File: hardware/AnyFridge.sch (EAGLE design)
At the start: 12 parts

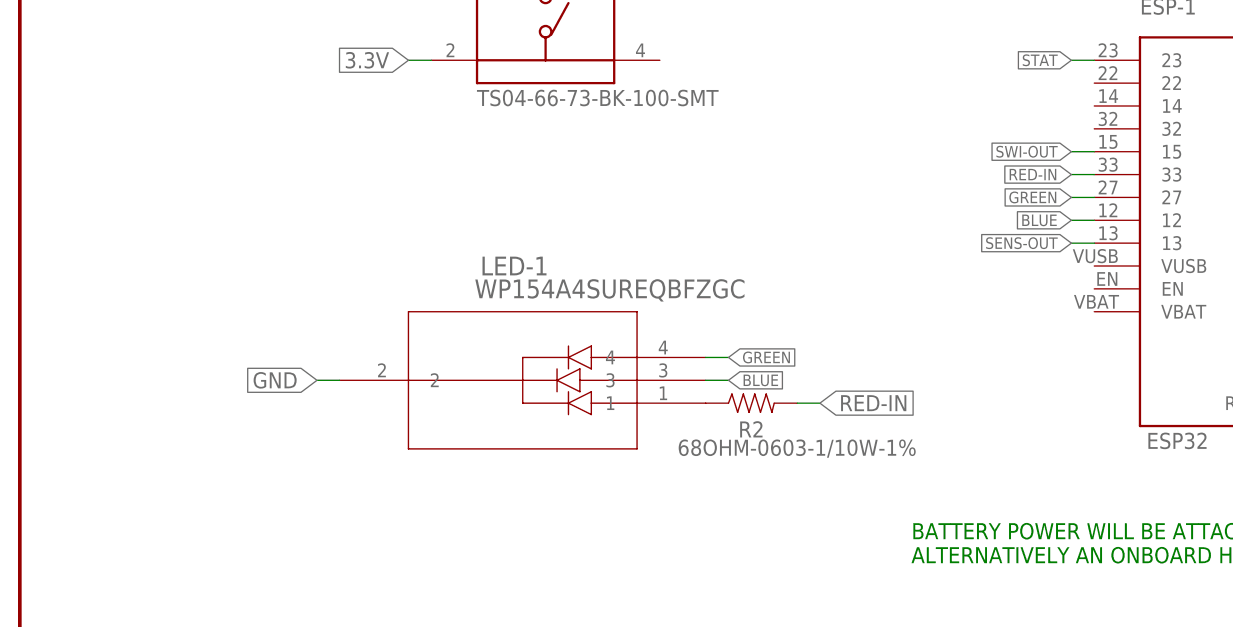
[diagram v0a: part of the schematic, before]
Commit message: Add Green and Blue resistors
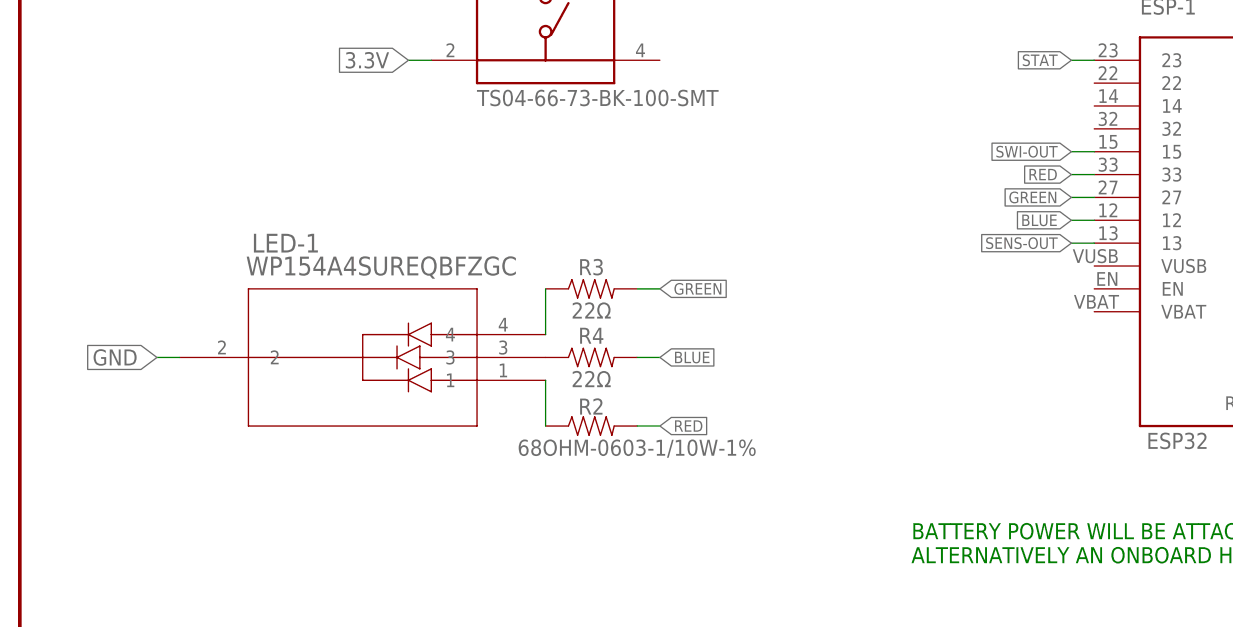
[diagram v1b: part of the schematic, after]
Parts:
- added R3, R4: 22Ω, SparkFun-Resistors:22OHM-0603-1/10W-1%
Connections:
- net RED-IN renamed RED
- new net N$2: LED-1.4, R3.1
- new net N$3: LED-1.3, R4.1
- net BLUE: now also R4.2; no longer LED-1.3
- net GREEN: now also R3.2; no longer LED-1.4
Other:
- moved on the sheet: LED-1, R2
